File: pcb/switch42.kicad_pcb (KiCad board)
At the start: 2 copper layers, 114.3 x 81 mm, 84 parts, among them J1 MJ-4PP-9, J2 Conn_01x03, SW1 SW_PUSH, SW10 SW_PUSH, SW11 SW_PUSH, SW12 SW_PUSH, SW13 SW_PUSH, SW14 SW_PUSH, SW15 SW_PUSH, SW16 SW_PUSH, SW17 SW_PUSH, SW18 SW_PUSH, SW19 SW_PUSH, SW2 SW_PUSH, SW20 SW_PUSH, SW21 SW_PUSH, SW22 SW_PUSH, SW23 SW_PUSH, SW24 SW_PUSH, SW25 SW_PUSH, SW3 SW_PUSH, SW4 SW_PUSH, SW5 SW_PUSH, SW6 SW_PUSH, SW7 SW_PUSH, SW8 SW_PUSH, SW9 SW_PUSH, U1 ProMicro

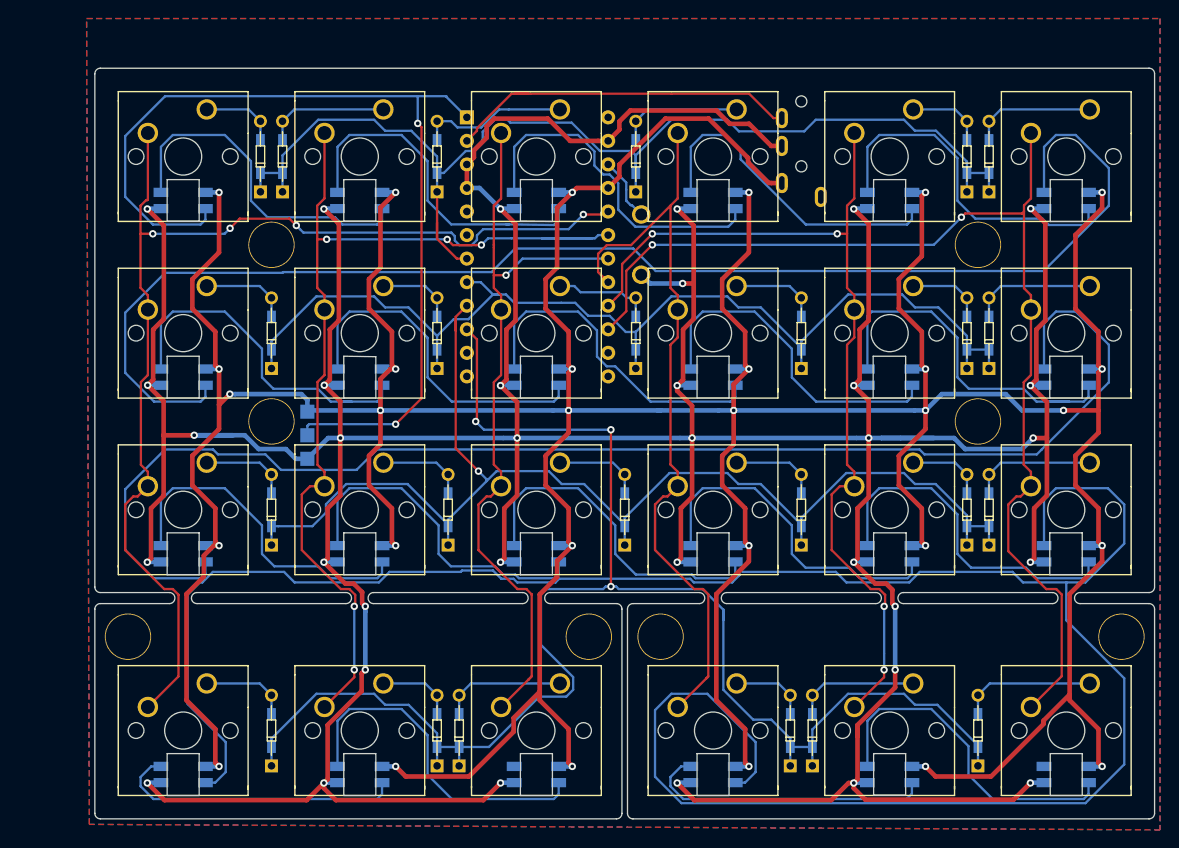
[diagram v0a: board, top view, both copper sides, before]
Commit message: KP-19 pcb
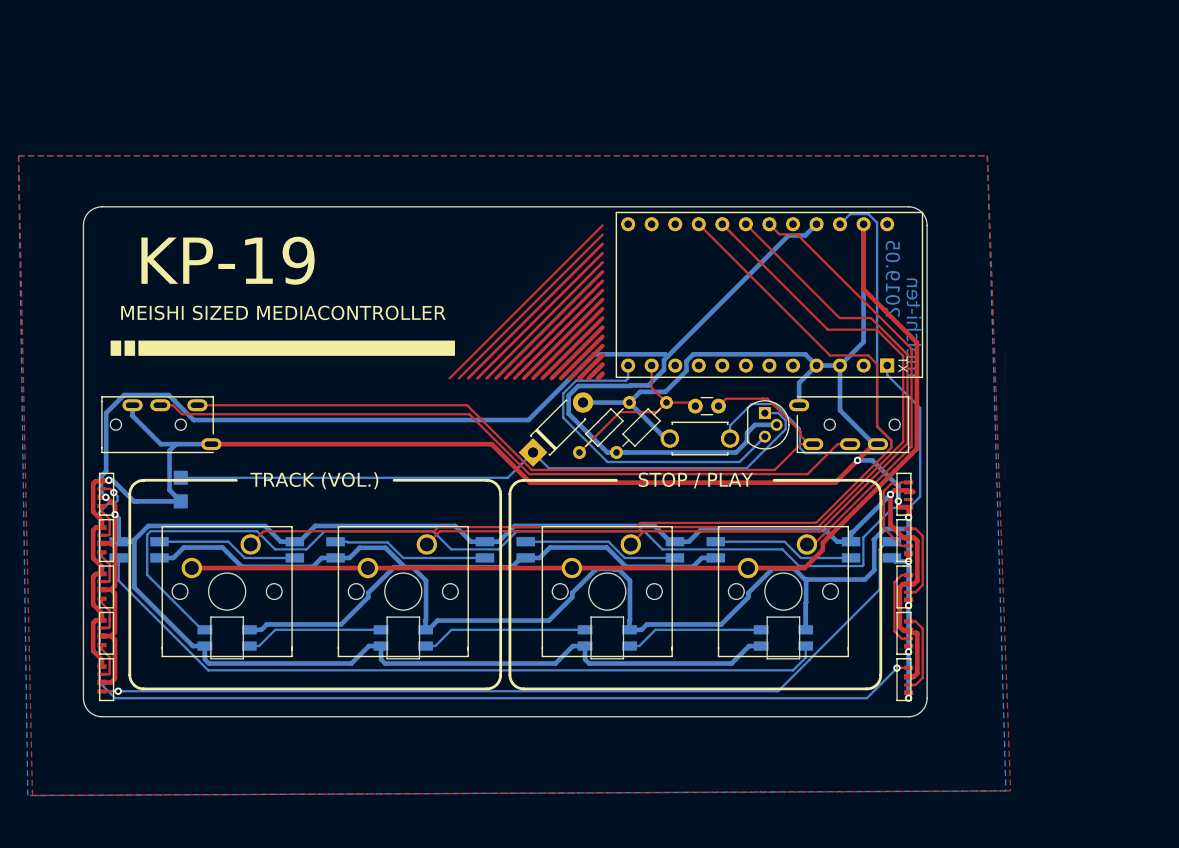
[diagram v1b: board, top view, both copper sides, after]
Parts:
- removed D10, D11, D12, D13, D14, D15, D16, D17, D18, D19, D2, D20, D21, D22, D23, D24, D3, D4, D5, D6, D7, D8, D9: D, phi-kbd-library:D_TH_SMD-irreversible
- removed L20, L21, L22, L23, L24: SK6812MINI, phi-kbd-library:SK6812MINI-irreversible
- removed Ref** (x8): Val**, kbd:HOLE
- removed SW10, SW11, SW12, SW13, SW14, SW15, SW16, SW17, SW18, SW19, SW20, SW21, SW22, SW23, SW24, SW25, SW3, SW6, SW8, SW9: SW_PUSH, phi-kbd-library:MX_1.00u-irreversible
- added C1: C, Capacitor_THT:C_Disc_D3.0mm_W1.6mm_P2.50mm, F.Cu at (116.0, 71.5)
- added G***: LOGO, paripi:Untitled, B.Cu at (63.2, 63.0)
- added J3: MJ-4PP-9, phi-kbd-library:MJ-4PP-9-irreversible, F.Cu at (139.0, 73.5)
- added Q1: Q_NPN_ECB, Package_TO_SOT_THT:TO-92, F.Cu at (123.5, 72.2)
- added R1: R, Resistor_THT:R_Axial_DIN0204_L3.6mm_D1.6mm_P7.62mm_Horizontal, F.Cu at (107.5, 76.5)
- added R2: R, Resistor_THT:R_Axial_DIN0204_L3.6mm_D1.6mm_P7.62mm_Horizontal, F.Cu at (103.5, 76.5)
- D1: footprint phi-kbd-library:D_TH_SMD-irreversible -> Diode_THT:D_DO-41_SOD81_P7.62mm_Horizontal
- J1: value MJ-4PP-9 -> Conn_01x02; footprint phi-kbd-library:MJ-4PP-9-irreversible -> phi-kbd-library:2pads
- J2: value Conn_01x03 -> MJ-4PP-9; footprint phi-kbd-library:StripLED-1mm-irreversible -> phi-kbd-library:MJ-4PP-9-irreversible; moved to F.Cu
- L1, L3, L5, L7, L9: footprint phi-kbd-library:SK6812MINI-irreversible -> phi-kbd-library:SK6812MINI-underglow-irreversible
- L10, L11, L12, L13, L14, L15, L2, L4, L6, L8: footprint phi-kbd-library:SK6812MINI-irreversible -> phi-kbd-library:SK6812SIDE-irreversible; moved to F.Cu
- SW1: footprint phi-kbd-library:ResetSW-irreversible -> phi-kbd-library:MX_1.00u-irreversible; moved to F.Cu
- SW7: footprint phi-kbd-library:MX_1.00u-irreversible -> phi-kbd-library:ResetSW-irreversible
- U1: moved to F.Cu
- moved J1 79.8 mm to (60.5, 80.5), turned to 0 degrees
- moved L17 70.6 mm to (84.5, 96.5), turned to 180 degrees
- moved SW5 66.5 mm to (125.5, 91.5)
- moved SW2 65.5 mm to (106.5, 91.5)
- moved SW1 58.3 mm to (65.5, 91.5), turned to 0 degrees
- moved L16 54.4 mm to (65.5, 96.5), turned to 180 degrees
- moved L9 52.2 mm to (135.0, 87.0), turned to 180 degrees
- moved L10 48.0 mm to (52.5, 81.0), turned to 90 degrees
- moved U1 47.4 mm to (140.5, 59.5), turned to 180 degrees
- moved L13 46.5 mm to (138.5, 91.0), turned to 270 degrees
- moved D1 43.4 mm to (98.5, 76.5), turned to 45 degrees
- moved L12 42.5 mm to (138.5, 96.0), turned to 270 degrees
- moved L11 41.9 mm to (138.5, 101.0), turned to 270 degrees
- moved L18 41.5 mm to (106.5, 96.5), turned to 180 degrees
- moved L5 40.8 mm to (95.5, 87.0), turned to 180 degrees
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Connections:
- D1 pad 1: row0 -> Net-(D1-Pad1)
- D1 pad 2: Net-(D1-Pad2) -> GND
- L1 pad 3: led -> underglow
- L11 pad 3: Net-(L11-Pad3) -> Net-(L10-Pad1)
- L12 pad 3: Net-(L12-Pad3) -> Net-(L11-Pad1)
- L13 pad 3: Net-(L13-Pad3) -> Net-(L12-Pad1)
- L14 pad 3: Net-(L10-Pad1) -> Net-(L13-Pad1)
- L15 pad 3: Net-(L11-Pad1) -> Net-(L14-Pad1)
- L16 pad 3: Net-(L16-Pad3) -> backlight
- L17 pad 3: Net-(L13-Pad1) -> Net-(L16-Pad1)
- L18 pad 3: Net-(L14-Pad1) -> Net-(L17-Pad1)
- L19 pad 1: Net-(L19-Pad1) -> underglow
- L19 pad 3: Net-(L15-Pad1) -> Net-(L18-Pad1)
- L2 pad 3: Net-(L2-Pad3) -> led
- L3 pad 3: Net-(L22-Pad1) -> Net-(L1-Pad1)
- L4 pad 3: Net-(L16-Pad3) -> Net-(L2-Pad1)
- L5 pad 3: Net-(L1-Pad1) -> Net-(L3-Pad1)
- L6 pad 1: Net-(L10-Pad3) -> Net-(L6-Pad1)
- L6 pad 3: Net-(L2-Pad1) -> Net-(L4-Pad1)
- L7 pad 1: Net-(L11-Pad3) -> Net-(L7-Pad1)
- L7 pad 3: Net-(L3-Pad1) -> Net-(L5-Pad1)
- L8 pad 1: Net-(L12-Pad3) -> Net-(L10-Pad3)
- L8 pad 3: Net-(L4-Pad1) -> Net-(L6-Pad1)
- L9 pad 1: Net-(L13-Pad3) -> led
- L9 pad 3: Net-(L5-Pad1) -> Net-(L7-Pad1)
- SW1 pad 1: reset -> GND
- SW1 pad 2: GND -> sw1
- SW2 pad 1: col0 -> GND
- SW2 pad 2: Net-(D1-Pad2) -> sw3
- SW4 pad 1: col0 -> GND
- SW4 pad 2: Net-(D3-Pad2) -> sw2
- SW5 pad 1: col0 -> GND
- SW5 pad 2: Net-(D4-Pad2) -> sw4
- SW7 pad 1: col1 -> reset
- SW7 pad 2: Net-(D6-Pad2) -> GND
- U1 pad 1: led -> backlight
- U1 pad 10: row3 -> Net-(U1-Pad10)
- U1 pad 11: Net-(U1-Pad11) -> audio
- U1 pad 12: Net-(U1-Pad12) -> vib
- U1 pad 15: col5 -> Net-(U1-Pad15)
- U1 pad 16: col4 -> sw1
- U1 pad 17: col3 -> sw2
- U1 pad 18: col2 -> sw3
- U1 pad 19: col1 -> sw4
- U1 pad 2: data -> Net-(U1-Pad2)
- U1 pad 20: col0 -> Net-(U1-Pad20)
- U1 pad 7: row0 -> Net-(U1-Pad7)
- U1 pad 8: row1 -> Net-(U1-Pad8)
- U1 pad 9: row2 -> Net-(U1-Pad9)
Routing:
- net Net-(L16-Pad3): track 253.0 -> 0.00 mm
- net (no net): track 0.00 -> 204.4 mm
- net VCC: track 569.6 -> 369.4 mm, vias 30 -> 3
- net row3: track 175.1 -> 0.00 mm, vias 3 -> 0
- net Net-(L22-Pad1): track 148.9 -> 0.00 mm
- net Net-(L2-Pad3): track 148.7 -> 0.00 mm
- net row2: track 132.8 -> 0.00 mm, vias 1 -> 0
- net col0: track 123.2 -> 0.00 mm, vias 4 -> 0
- net row0: track 122.5 -> 0.00 mm
- net backlight: track 0.00 -> 121.8 mm
- net col5: track 121.5 -> 0.00 mm, vias 2 -> 0
- net row1: track 115.9 -> 0.00 mm
- net sw1: track 0.00 -> 108.8 mm
- net col1: track 107.5 -> 0.00 mm, vias 5 -> 0
- net col4: track 100.2 -> 0.00 mm, vias 4 -> 0
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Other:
- board size 114.3 x 81 mm -> 91 x 55 mm
- board text added: "100K"
- board text added: "10uF"
- board text added: "1N4007"
- board text added: "2019.05"
- board text added: "2SC1815"
- board text added: "4-MX Switches"
- board text added: "4-SK6812mini"
- board text added: "5-SK6812Side"
- board text added: "5-SK6812mini"
- board text added: "GitHub: https://github.com/zk-phi Twitter: https://twitter.com/zk_phi"
- board text added: "KP-19"
- board text added: "MEISHI SIZED MEDIACONTROLLER"
- board text added: "MJ-4PP-9"
- board text added: "Pro Micro"
- board text added: "STOP / PLAY"
- board text added: "Software Engineer"
- board text added: "TRACK (VOL.)"
- board text added: "TVBP06"
- board text added: "Vib"
- board text added: "meishi-ten"
- board text added: "zk_phi"
- board text removed: "* switch42 v0.3 designed by @zk_phi *"
- board text removed: "DIN"
- board text removed: "L"
- board text removed: "R"
- board text removed: "VCC"
